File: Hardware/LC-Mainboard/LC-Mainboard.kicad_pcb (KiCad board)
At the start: 2 copper layers, 100.5 x 86 mm, 44 parts, among them J1 Raspberry_Pi, J2 Charge Controller, J3 I²C_conn, J4 Beacon_conn, J5 Star_Motor_conn, J6 Port_Motor_conn, J7 DC_conn, J8 PTT_conn, U1 MAX3232IDW

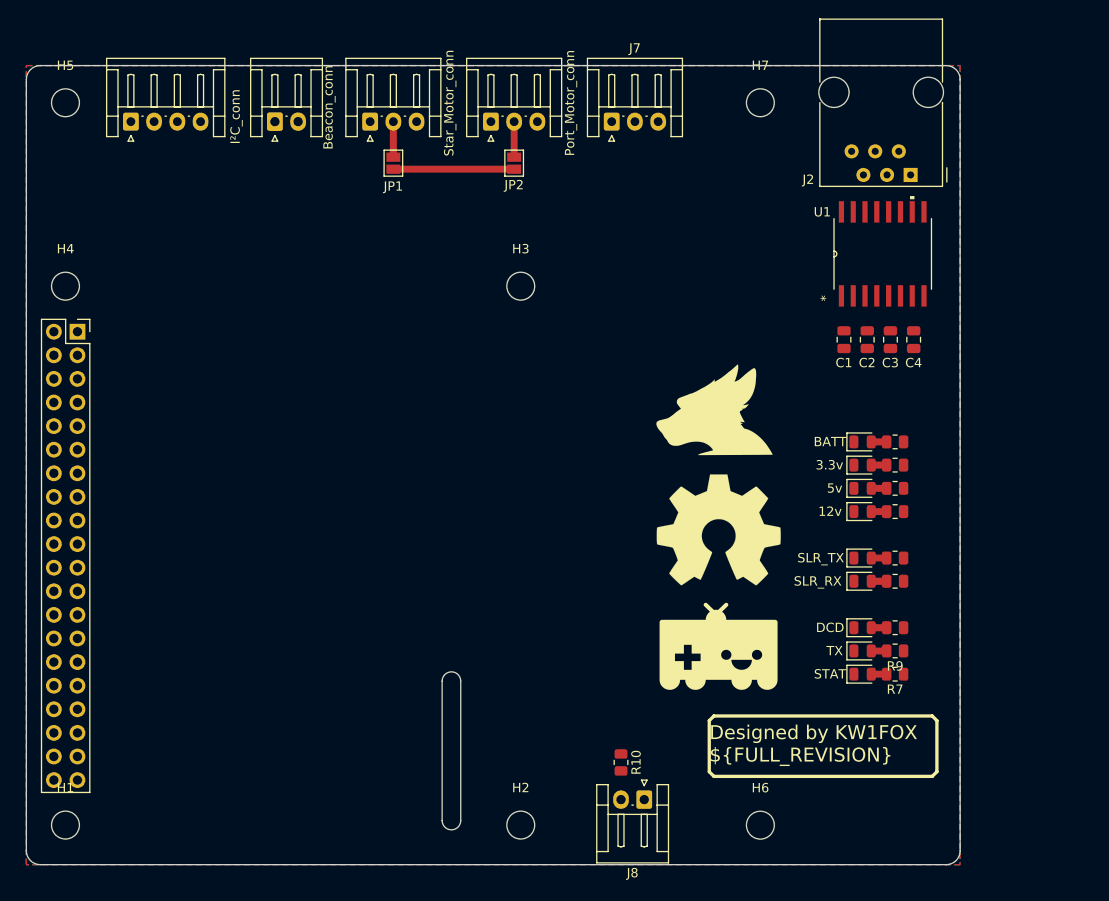
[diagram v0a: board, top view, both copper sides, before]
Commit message: Add a bunch of stuff
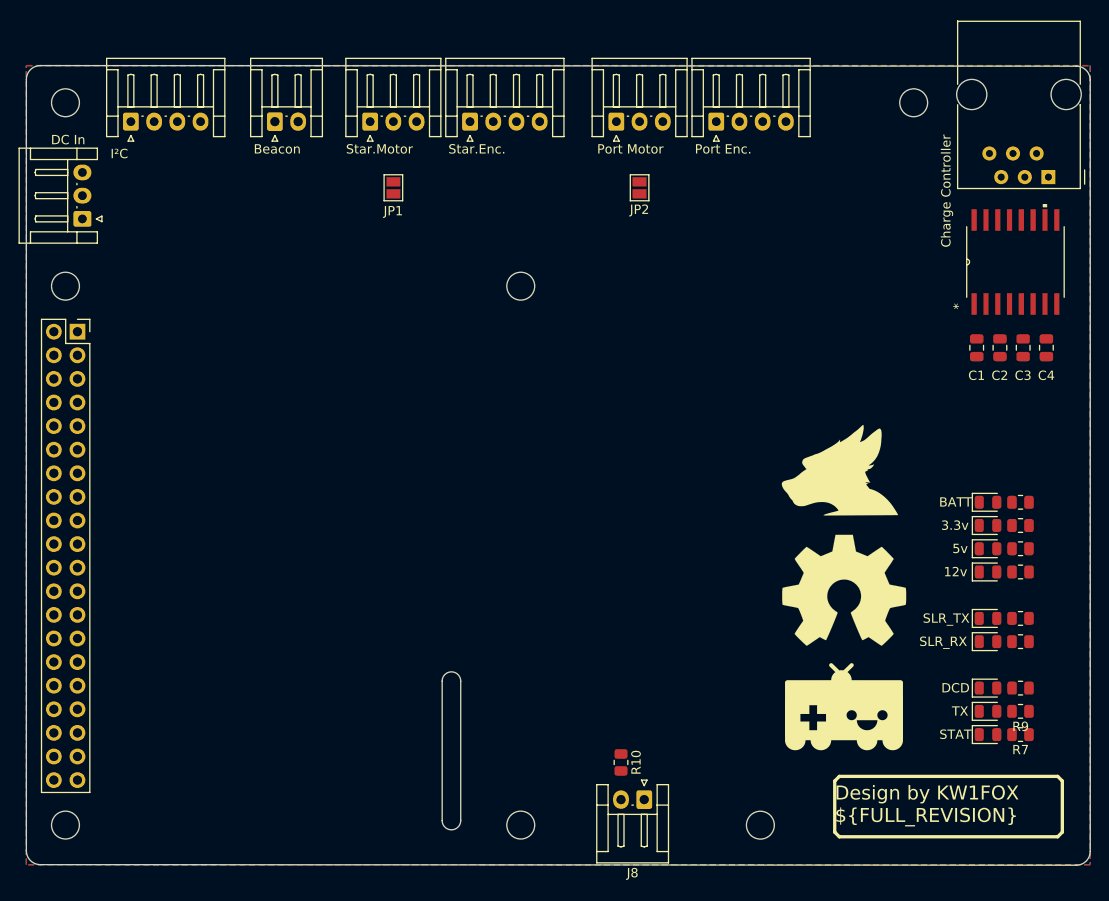
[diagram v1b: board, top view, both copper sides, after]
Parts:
- added J10: Port Enc., Connector_JST:JST_EH_S4B-EH_1x04_P2.50mm_Horizontal, F.Cu at (177.8, 54.5)
- added J9: Star.Enc., Connector_JST:JST_EH_S4B-EH_1x04_P2.50mm_Horizontal, F.Cu at (151.2, 54.5)
- J3: value I²C_conn -> I²C
- J4: value Beacon_conn -> Beacon
- J5: value Star_Motor_conn -> Star.Motor
- J6: value Port_Motor_conn -> Port Motor
- J7: value DC_conn -> DC In
- J8: value PTT_conn -> PTT
- moved J7 57.9 mm to (109.5, 65.0), turned to 90 degrees
- moved H7 16.5 mm to (199.0, 52.5)
- moved D1 15.0 mm to (207.0, 110.5)
- moved D2 15.0 mm to (207.0, 108.0)
- moved D3 15.0 mm to (207.0, 103.0)
- moved D4 15.0 mm to (207.0, 100.5)
- moved D5 15.0 mm to (207.0, 98.0)
- moved D6 15.0 mm to (207.0, 115.5)
- moved D7 15.0 mm to (207.0, 120.5)
- moved D8 15.0 mm to (207.0, 95.5)
- moved D9 15.0 mm to (207.0, 118.0)
- moved G*** 15.0 mm to (191.0, 92.0)
- moved G*** 15.0 mm to (191.5, 117.5)
- moved R1 15.0 mm to (210.5, 110.5)
- moved R2 15.0 mm to (210.5, 108.0)
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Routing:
- net +5V: track 13.0 -> 0.00 mm
- net Net-(J6-Pad2): track 3.82 -> 0.00 mm
- net Net-(J5-Pad2): track 3.82 -> 0.00 mm
- net Net-(D9-Pad2): track 1.65 -> 0.00 mm
- net Net-(D8-Pad2): track 1.65 -> 0.00 mm
- net Net-(D7-Pad2): track 1.65 -> 0.00 mm
- net Net-(D6-Pad2): track 1.65 -> 0.00 mm
- net Net-(D5-Pad2): track 1.65 -> 0.00 mm
- net Net-(D4-Pad2): track 1.65 -> 0.00 mm
- net Net-(D3-Pad2): track 1.65 -> 0.00 mm
- net Net-(D2-Pad2): track 1.65 -> 0.00 mm
- net Net-(D1-Pad2): track 1.65 -> 0.00 mm
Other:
- board size 100.5 x 86 mm -> 114.5 x 86.1 mm
- board text added: "Design by KW1FOX ${FULL_REVISION}"
- board text removed: "Designed by KW1FOX ${FULL_REVISION}"

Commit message: Make a v1.0 hardware release (#2)
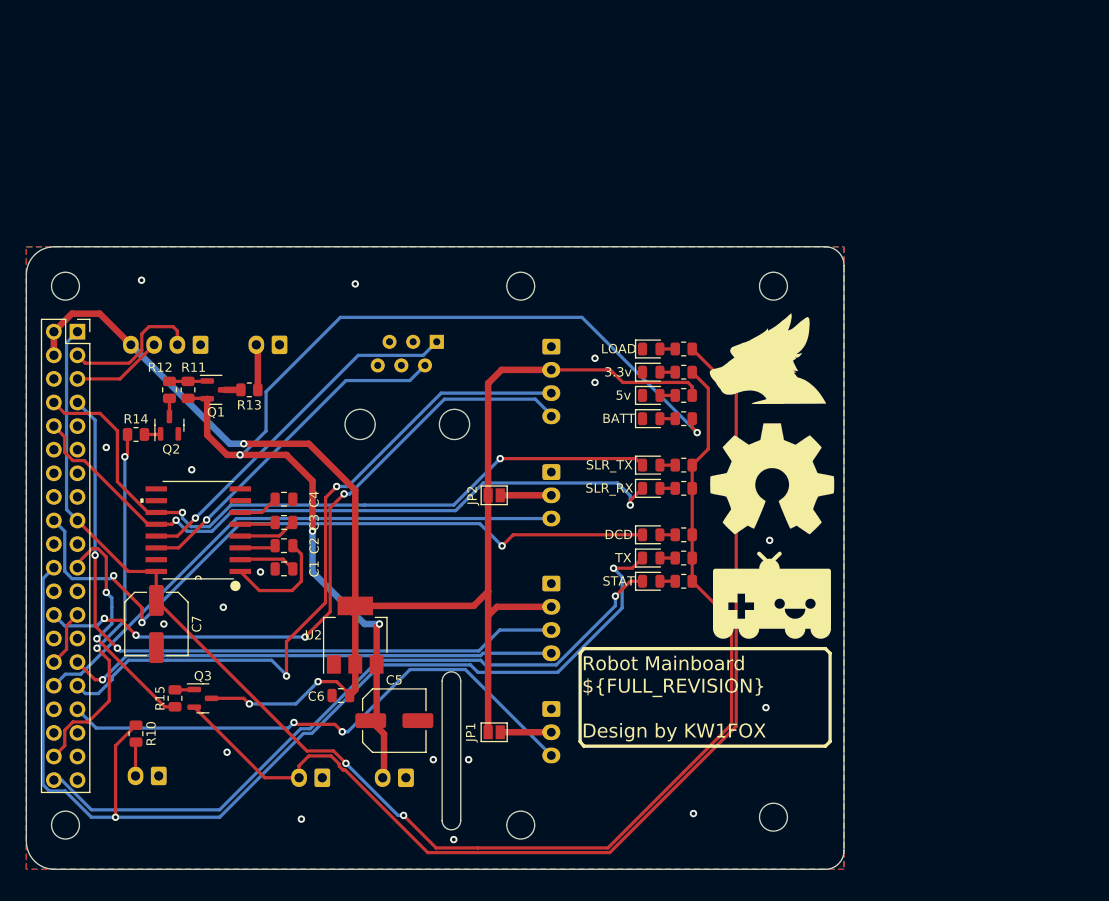
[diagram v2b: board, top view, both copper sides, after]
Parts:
- removed the H5 at (107.7, 52.5)
- added C5: 10μf, Capacitor_SMD:C_Elec_6.3x5.4, F.Cu at (143.1, 119.0)
- added C6: 0.1μf, Capacitor_SMD:C_0805_2012Metric, F.Cu at (137.3, 116.3)
- added C7: 10μf, Capacitor_SMD:C_Elec_6.3x5.4, F.Cu at (117.5, 108.6)
- added J11: Load En., Connector_JST:JST_XH_S2B-XH-A_1x02_P2.50mm_Horizontal, B.Cu at (135.3, 125.2)
- added Q1: MMBT3906, Package_TO_SOT_SMD:SOT-23, F.Cu at (123.9, 83.4)
- added Q2: MMBT3904, Package_TO_SOT_SMD:SOT-23, F.Cu at (118.9, 87.2)
- added Q3: MMBT3904, Package_TO_SOT_SMD:SOT-23, F.Cu at (122.5, 116.6)
- added R11: 47K, Resistor_SMD:R_0805_2012Metric, F.Cu at (120.9, 83.4)
- added R12: 1K, Resistor_SMD:R_0805_2012Metric, F.Cu at (118.9, 83.4)
- added R13: 47R, Resistor_SMD:R_0805_2012Metric, F.Cu at (127.5, 83.4)
- added R14: 1K, Resistor_SMD:R_0805_2012Metric, F.Cu at (115.3, 88.2)
- added R15: 1K, Resistor_SMD:R_0805_2012Metric, F.Cu at (119.5, 116.6)
- added U2: NCP1117-12_SOT223, Package_TO_SOT_SMD:SOT-223-3_TabPin2, F.Cu at (138.9, 109.8)
- D3: value 12v -> BATT
- D8: value BATT -> LOAD
- J10, J3, J9: footprint Connector_JST:JST_EH_S4B-EH_1x04_P2.50mm_Horizontal -> Connector_JST:JST_XH_S4B-XH-A_1x04_P2.50mm_Horizontal; moved to B.Cu
- J2: moved to B.Cu
- J4, J8: footprint Connector_JST:JST_EH_S2B-EH_1x02_P2.50mm_Horizontal -> Connector_JST:JST_XH_S2B-XH-A_1x02_P2.50mm_Horizontal; moved to B.Cu
- J5, J6: footprint Connector_JST:JST_EH_S3B-EH_1x03_P2.50mm_Horizontal -> Connector_JST:JST_XH_S3B-XH-A_1x03_P2.50mm_Horizontal; moved to B.Cu
- J7: footprint Connector_JST:JST_EH_S3B-EH_1x03_P2.50mm_Horizontal -> Connector_JST:JST_XH_S2B-XH-A_1x02_P2.50mm_Horizontal; moved to B.Cu
- R1, R2, R5, R6, R7, R9: value 100k -> 100R
- R10: value math -> 470R
- R3, R8: value math -> 1K
- R4: value math -> 220R
- moved U1 92.6 mm to (122.0, 98.5), turned to 180 degrees
- moved C4 83.7 mm to (131.2, 95.2), turned to 0 degrees
- moved C3 81.7 mm to (131.2, 97.7), turned to 180 degrees
- moved C2 79.9 mm to (131.2, 100.2), turned to 180 degrees
- moved C1 78.3 mm to (131.2, 102.7), turned to 180 degrees
- moved J7 69.5 mm to (144.3, 125.2), turned to 180 degrees
- moved J2 68.2 mm to (147.7, 78.2)
- moved J5 66.2 mm to (160.0, 117.8), turned to -90 degrees
- moved JP1 59.6 mm to (153.8, 120.2), turned to 180 degrees
- moved J8 52.3 mm to (117.8, 125.0)
- moved R10 52.3 mm to (115.3, 120.4)
- moved J9 50.5 mm to (160.0, 104.2), turned to -90 degrees
- moved D1 39.8 mm to (170.8, 94.0)
- moved D2 39.8 mm to (170.8, 91.5)
- moved D3 39.8 mm to (170.8, 86.5)
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- renumbered H7 to H5
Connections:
- C1 pad 1: +3V3 -> Net-(C1-Pad1)
- C1 pad 2: Net-(C1-Pad2) -> GND
- D9 pad 1: TX_LED -> PTT
- J1 pad 21: unconnected-(J1-Pad21) -> LOAD_EN_Pi
- J1 pad 26: unconnected-(J1-Pad26) -> PORT_ENC_B
- J1 pad 29: unconnected-(J1-Pad29) -> STAR_ENC_B
- J1 pad 31: unconnected-(J1-Pad31) -> PORT_ENC_A
- J1 pad 38: unconnected-(J1-Pad38) -> BCON_LED
- J1 pad 7: unconnected-(J1-Pad7) -> STAR_ENC_A
- J4 pad 2: unconnected-(J4-Pad2) -> BCON_LOAD
- R8 pad 1: +12VA -> LOAD_EN
- U1 pad 2: Net-(C1-Pad2) -> Net-(C1-Pad1)
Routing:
- net +5V: track 0.00 -> 166.7 mm, vias 0 -> 3
- net +3V3: track 0.00 -> 154.7 mm, vias 0 -> 2
- net +12V: track 0.00 -> 121.0 mm, vias 0 -> 4
- net PTT: track 0.00 -> 116.7 mm, vias 0 -> 2
- net LOAD_EN: track 0.00 -> 115.9 mm
- net DCD_LED: track 0.00 -> 77.8 mm, vias 0 -> 3
- net STAR_ENC_A: track 0.00 -> 76.0 mm, vias 0 -> 2
- net STAT_LED: track 0.00 -> 75.9 mm, vias 0 -> 1
- net PI_TX: track 0.00 -> 75.8 mm, vias 0 -> 2
- net PORT_ENC_A: track 0.00 -> 75.2 mm, vias 0 -> 2
- net PI_RX: track 0.00 -> 74.1 mm, vias 0 -> 2
- net PORT_ENC_B: track 0.00 -> 73.2 mm, vias 0 -> 4
- net PORT_PWM: track 0.00 -> 61.0 mm
- net STAR_PWM: track 0.00 -> 59.1 mm, vias 0 -> 2
- net STAR_ENC_B: track 0.00 -> 53.0 mm, vias 0 -> 1
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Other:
- board size 114.5 x 86.1 mm -> 88 x 67 mm
- board text added: "5V"
- board text added: "BAT"
- board text added: "ENC.A"
- board text added: "ENC.B"
- board text added: "PWM"
- board text added: "RELAY"
- board text added: "Robot Mainboard ${FULL_REVISION} Design by KW1FOX"
- board text added: "SCL"
- board text added: "SDA"
- board text removed: "Design by KW1FOX ${FULL_REVISION}"
